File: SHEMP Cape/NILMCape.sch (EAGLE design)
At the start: 88 parts, among them U1 ADS8568_PM_64, U10 SI8663BC-B-IS1, U11 SI8663BC-B-IS1, U12 SI8663BC-B-IS1, U13 SI8663BC-B-IS1, U14 SN74CBT16390_DGG, U2 ACS756KCA-050B-PFF-T, U3 SI8663BC-B-IS1, U4 SN74CBT16390_DGG, U5 TPS84250_RKG_41, U6 TPS7A3301_RGW_20, U7 LP2950-33_KVU_3, U8 SI8663BC-B-IS1, U9 TL074_PW_14

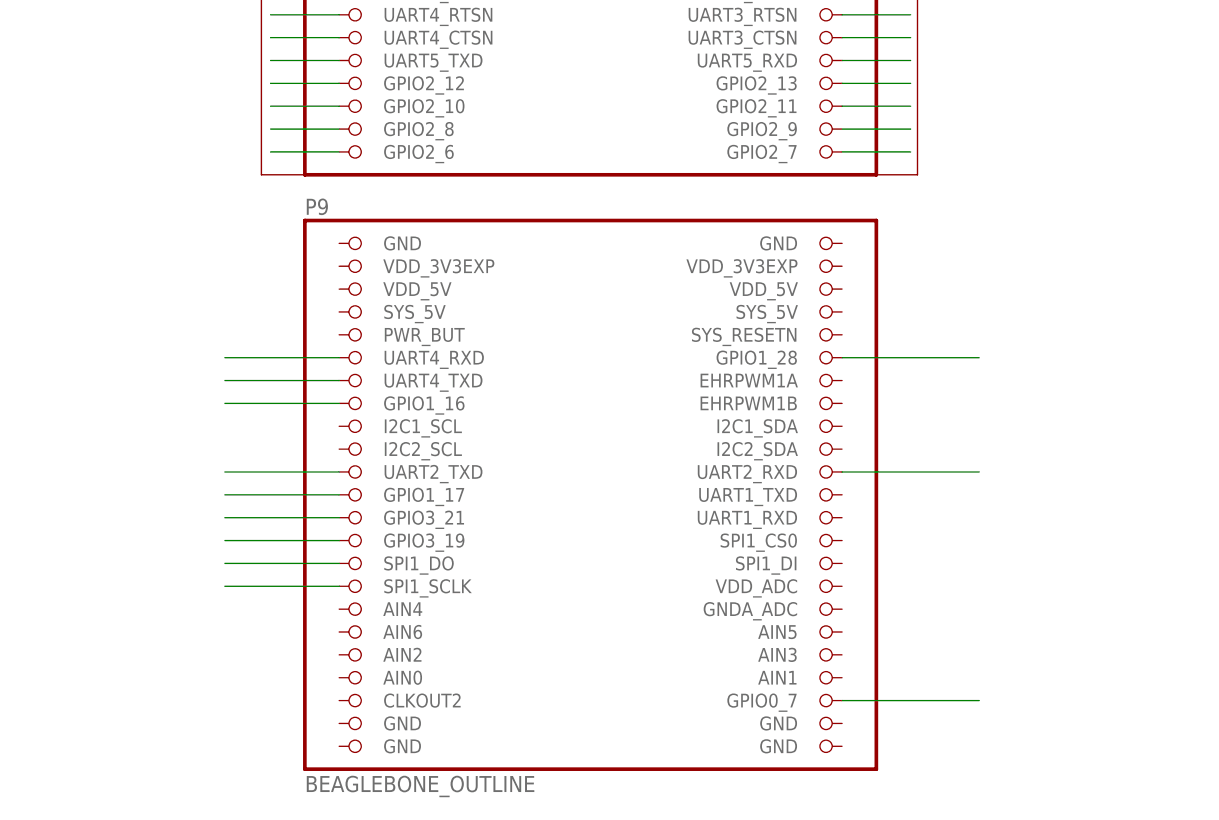
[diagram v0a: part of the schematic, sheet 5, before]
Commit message: More schematic capture work.
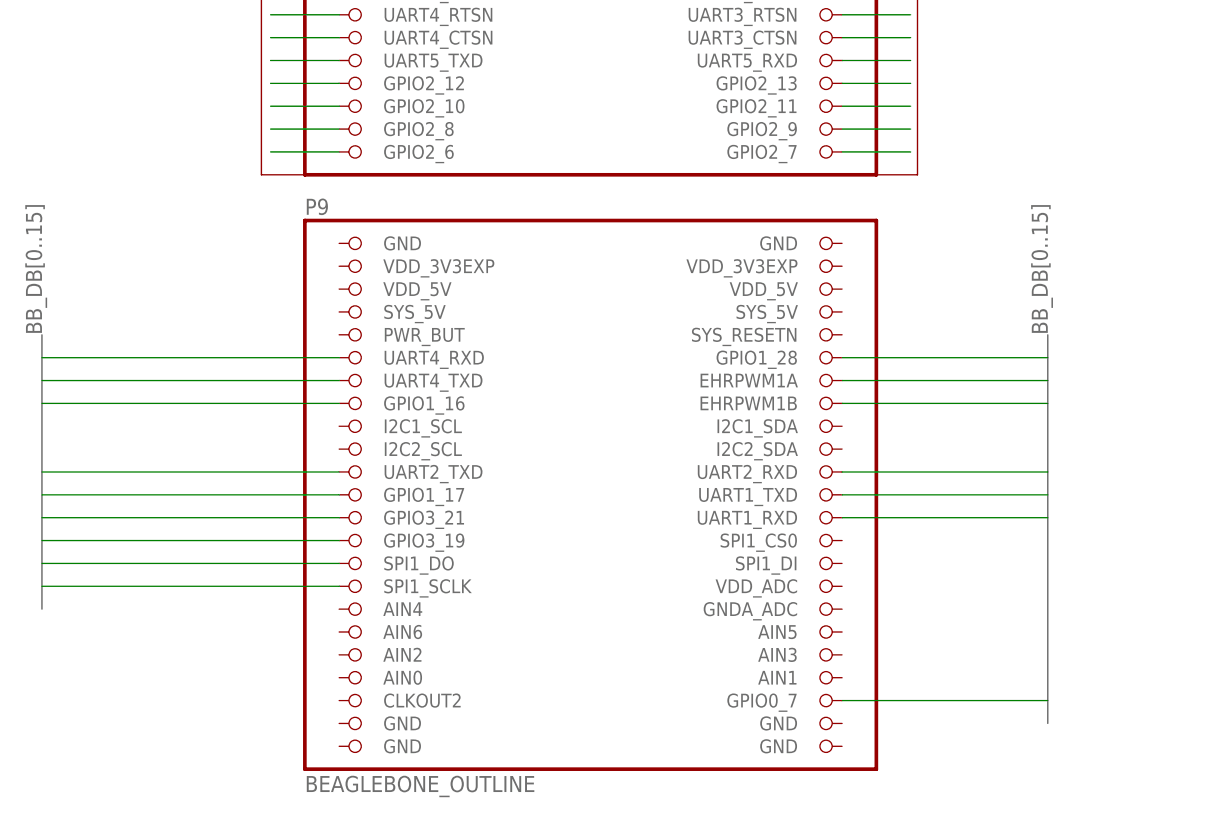
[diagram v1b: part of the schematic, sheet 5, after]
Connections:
- removed net N$100: U$1.SPI1_SCLK
- removed net N$86: U$1.GPIO1_28
- removed net N$87: U$1.GPIO3_19
- removed net N$88: U$1.GPIO3_21
- removed net N$89: U$1.GPIO1_17
- removed net N$93: U$1.GPIO1_16
- removed net N$94: U$1.GPIO0_7
- removed net N$95: U$1.UART2_TXD
- removed net N$96: U$1.UART2_RXD
- removed net N$97: U$1.UART4_RXD
- removed net N$98: U$1.UART4_TXD
- removed net N$99: U$1.SPI1_DO
- net BB_DB0: now also U$1.UART4_RXD
- net BB_DB1: now also U$1.UART4_TXD
- net BB_DB10: now also U$1.EHRPWM1A
- net BB_DB11: now also U$1.EHRPWM1B
- net BB_DB12: now also U$1.UART2_RXD
- net BB_DB13: now also U$1.UART1_TXD
- net BB_DB14: now also U$1.UART1_RXD
- net BB_DB15: now also U$1.GPIO0_7
- net BB_DB2: now also U$1.GPIO1_16
- net BB_DB3: now also U$1.UART2_TXD
- net BB_DB4: now also U$1.GPIO1_17
- net BB_DB5: now also U$1.GPIO3_21
- net BB_DB6: now also U$1.GPIO3_19
- net BB_DB7: now also U$1.SPI1_DO
- net BB_DB8: now also U$1.SPI1_SCLK
- net BB_DB9: now also U$1.GPIO1_28
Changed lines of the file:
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@@
 </instances>
 <busses>
+<bus name="BB_DB[0..15]">
+<segment>
+<wire x1="154.94" y1="137.16" x2="154.94" y2="106.68" width="0.762" layer="92"/>
+<label x="154.94" y="137.16" size="1.778" layer="95" rot="R90"/>
+</segment>
+<segment>
+<wire x1="266.7" y1="137.16" x2="266.7" y2="93.98" width="0.762" layer="92"/>
+<label x="266.7" y="137.16" size="1.778" layer="95" rot="R90"/>
+</segment>
+</bus>
 </busses>
 <nets>
@@
 </segment>
 </net>
-<net name="N$86" class="0">
-<segment>
-<pinref part="U$1" gate="G$1" pin="GPIO1_28"/>
-<wire x1="243.84" y1="134.62" x2="259.08" y2="134.62" width="0.1524" layer="91"/>
-</segment>
-</net>
-<net name="N$87" class="0">
-<segment>
-<pinref part="U$1" gate="G$1" pin="GPIO3_19"/>
-<wire x1="187.96" y1="114.3" x2="175.26" y2="114.3" width="0.1524" layer="91"/>
-</segment>
-</net>
-<net name="N$88" class="0">
-<segment>
-<pinref part="U$1" gate="G$1" pin="GPIO3_21"/>
-<wire x1="187.96" y1="116.84" x2="175.26" y2="116.84" width="0.1524" layer="91"/>
-</segment>
-</net>
-<net name="N$89" class="0">
-<segment>
-<pinref part="U$1" gate="G$1" pin="GPIO1_17"/>
-<wire x1="187.96" y1="119.38" x2="175.26" y2="119.38" width="0.1524" layer="91"/>
-</segment>
-</net>
 <net name="N$77" class="0">
 <segment>
@@
 </segment>
 </net>
-<net name="N$93" class="0">
+<net name="BB_DB0" class="0">
+<segment>
+<pinref part="U$1" gate="G$1" pin="UART4_RXD"/>
+<wire x1="154.94" y1="134.62" x2="187.96" y2="134.62" width="0.1524" layer="91"/>
+</segment>
+</net>
+<net name="BB_DB1" class="0">
+<segment>
+<pinref part="U$1" gate="G$1" pin="UART4_TXD"/>
+<wire x1="154.94" y1="132.08" x2="187.96" y2="132.08" width="0.1524" layer="91"/>
+</segment>
+</net>
+<net name="BB_DB2" class="0">
 <segment>
 <pinref part="U$1" gate="G$1" pin="GPIO1_16"/>
-<wire x1="187.96" y1="129.54" x2="175.26" y2="129.54" width="0.1524" layer="91"/>
-</segment>
-</net>
-<net name="N$94" class="0">
+<wire x1="154.94" y1="129.54" x2="187.96" y2="129.54" width="0.1524" layer="91"/>
+</segment>
+</net>
+<net name="BB_DB3" class="0">
+<segment>
+<pinref part="U$1" gate="G$1" pin="UART2_TXD"/>
+<wire x1="154.94" y1="121.92" x2="187.96" y2="121.92" width="0.1524" layer="91"/>
+</segment>
+</net>
+<net name="BB_DB4" class="0">
+<segment>
+<pinref part="U$1" gate="G$1" pin="GPIO1_17"/>
+<wire x1="154.94" y1="119.38" x2="187.96" y2="119.38" width="0.1524" layer="91"/>
+</segment>
+</net>
+<net name="BB_DB5" class="0">
+<segment>
+<pinref part="U$1" gate="G$1" pin="GPIO3_21"/>
+<wire x1="154.94" y1="116.84" x2="187.96" y2="116.84" width="0.1524" layer="91"/>
+</segment>
+</net>
+<net name="BB_DB6" class="0">
+<segment>
+<pinref part="U$1" gate="G$1" pin="GPIO3_19"/>
+<wire x1="154.94" y1="114.3" x2="187.96" y2="114.3" width="0.1524" layer="91"/>
+</segment>
+</net>
+<net name="BB_DB7" class="0">
+<segment>
+<pinref part="U$1" gate="G$1" pin="SPI1_DO"/>
+<wire x1="154.94" y1="111.76" x2="187.96" y2="111.76" width="0.1524" layer="91"/>
+</segment>
+</net>
+<net name="BB_DB8" class="0">
+<segment>
+<pinref part="U$1" gate="G$1" pin="SPI1_SCLK"/>
+<wire x1="154.94" y1="109.22" x2="187.96" y2="109.22" width="0.1524" layer="91"/>
+</segment>
+</net>
+<net name="BB_DB9" class="0">
+<segment>
+<pinref part="U$1" gate="G$1" pin="GPIO1_28"/>
+<wire x1="243.84" y1="134.62" x2="266.7" y2="134.62" width="0.1524" layer="91"/>
+</segment>
+</net>
+<net name="BB_DB10" class="0">
+<segment>
+<pinref part="U$1" gate="G$1" pin="EHRPWM1A"/>
+<wire x1="243.84" y1="132.08" x2="266.7" y2="132.08" width="0.1524" layer="91"/>
+</segment>
+</net>
+<net name="BB_DB11" class="0">
+<segment>
+<pinref part="U$1" gate="G$1" pin="EHRPWM1B"/>
+<wire x1="243.84" y1="129.54" x2="266.7" y2="129.54" width="0.1524" layer="91"/>
+</segment>
+</net>
+<net name="BB_DB12" class="0">
+<segment>
+<pinref part="U$1" gate="G$1" pin="UART2_RXD"/>
+<wire x1="243.84" y1="121.92" x2="266.7" y2="121.92" width="0.1524" layer="91"/>
+</segment>
+</net>
+<net name="BB_DB13" class="0">
+<segment>
+<pinref part="U$1" gate="G$1" pin="UART1_TXD"/>
+<wire x1="243.84" y1="119.38" x2="266.7" y2="119.38" width="0.1524" layer="91"/>
+</segment>
+</net>
+<net name="BB_DB14" class="0">
+<segment>
+<pinref part="U$1" gate="G$1" pin="UART1_RXD"/>
+<wire x1="243.84" y1="116.84" x2="266.7" y2="116.84" width="0.1524" layer="91"/>
+</segment>
+</net>
+<net name="BB_DB15" class="0">
 <segment>
 <pinref part="U$1" gate="G$1" pin="GPIO0_7"/>
-<wire x1="243.84" y1="96.52" x2="259.08" y2="96.52" width="0.1524" layer="91"/>
-</segment>
-</net>
-<net name="N$95" class="0">
-<segment>
-<pinref part="U$1" gate="G$1" pin="UART2_TXD"/>
-<wire x1="187.96" y1="121.92" x2="175.26" y2="121.92" width="0.1524" layer="91"/>
-</segment>
-</net>
-<net name="N$96" class="0">
-<segment>
-<pinref part="U$1" gate="G$1" pin="UART2_RXD"/>
-<wire x1="243.84" y1="121.92" x2="259.08" y2="121.92" width="0.1524" layer="91"/>
-</segment>
-</net>
-<net name="N$97" class="0">
-<segment>
-<pinref part="U$1" gate="G$1" pin="UART4_RXD"/>
-<wire x1="187.96" y1="134.62" x2="175.26" y2="134.62" width="0.1524" layer="91"/>
-</segment>
-</net>
-<net name="N$98" class="0">
-<segment>
-<pinref part="U$1" gate="G$1" pin="UART4_TXD"/>
-<wire x1="187.96" y1="132.08" x2="175.26" y2="132.08" width="0.1524" layer="91"/>
-</segment>
-</net>
-<net name="N$99" class="0">
-<segment>
-<pinref part="U$1" gate="G$1" pin="SPI1_DO"/>
-<wire x1="187.96" y1="111.76" x2="175.26" y2="111.76" width="0.1524" layer="91"/>
-</segment>
-</net>
-<net name="N$100" class="0">
-<segment>
-<pinref part="U$1" gate="G$1" pin="SPI1_SCLK"/>
-<wire x1="187.96" y1="109.22" x2="175.26" y2="109.22" width="0.1524" layer="91"/>
-</segment>
-</net>
+<wire x1="243.84" y1="96.52" x2="266.7" y2="96.52" width="0.1524" layer="91"/>
+</segment>
+</net>
